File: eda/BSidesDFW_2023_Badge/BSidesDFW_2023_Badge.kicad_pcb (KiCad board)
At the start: 2 copper layers, 50 x 63 mm, 12 parts

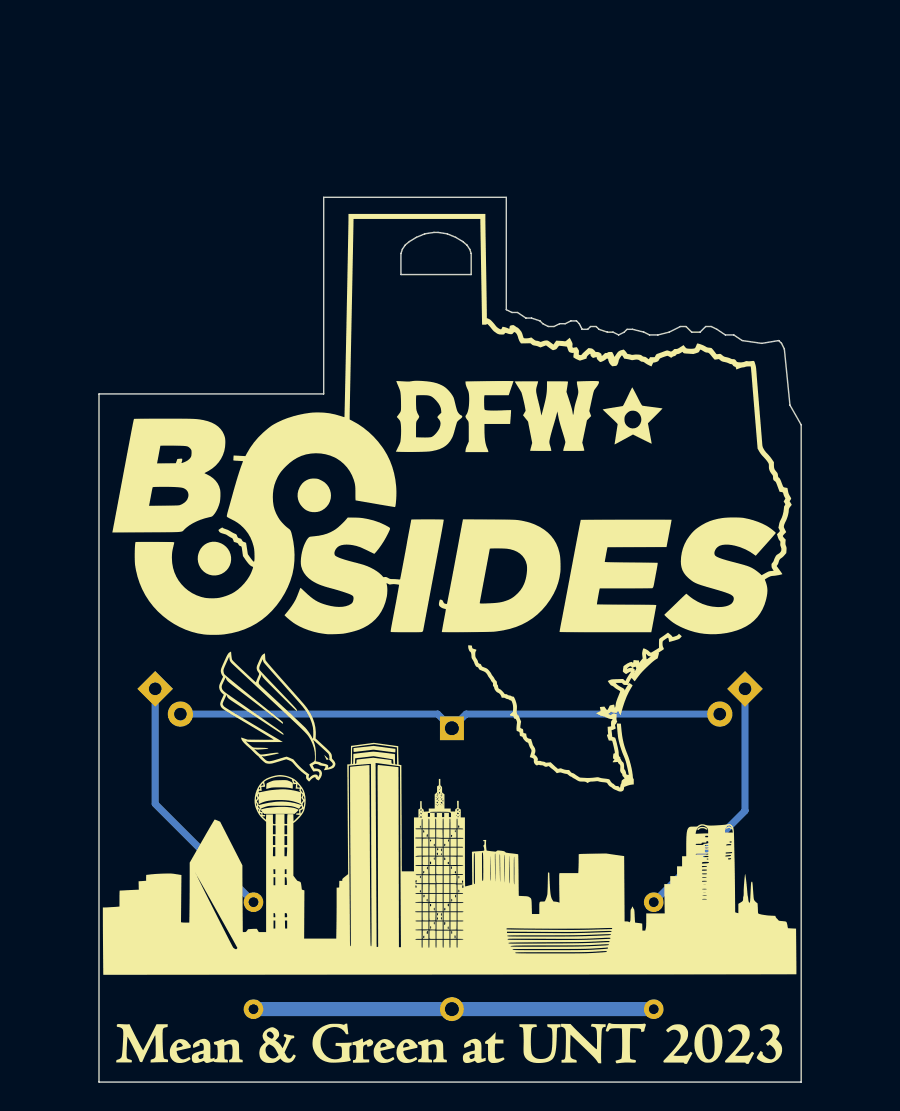
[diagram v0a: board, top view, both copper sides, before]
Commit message: final pcb design
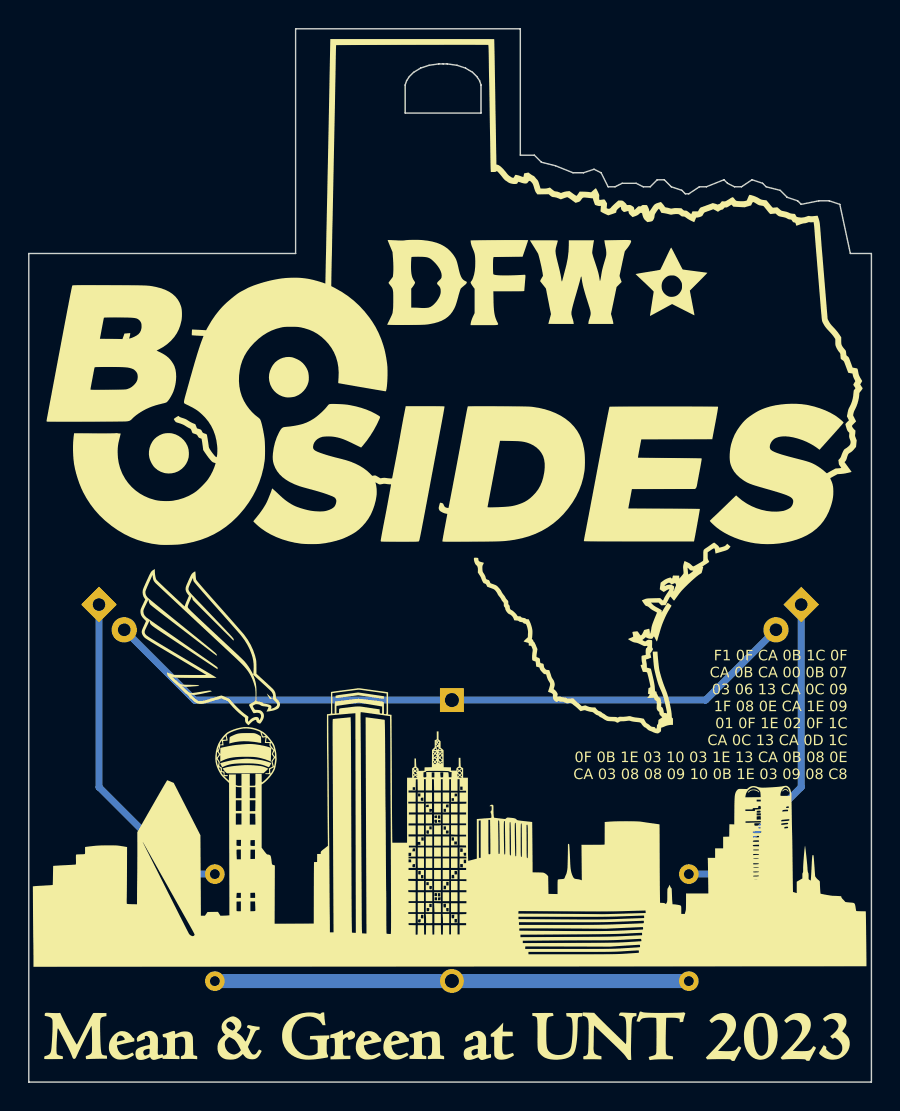
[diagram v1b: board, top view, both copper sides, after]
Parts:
- added G***: bsilk-scrappy, 0_local:0_UNT_old_scrappy_bsilk_1, F.Cu at (91.6, 127.6)
- BT1: footprint 0_local:BatteryHolder_CR2032-BS-2-1_Front_backsilk -> 0_local:BatteryHolder_CR2032-BS-2-1_Back_backsilk
- D1, D2: footprint 0_local:LED_D5.0mm-2_backsilk -> 0_local:LED_D5.0mm-2_backsilk_3Dback_horiz
- G***: footprint 0_alt_bier:logo-alt_bier-1100dpi-8x21mm-back -> 0_alt_bier:logo-alt_bier-900dpi-10x25mm-back
- G001: renamed from G002; footprint 0_local:0_BsidesDFW_top_fsilk_2 -> 0_local:0_BsidesDFW_top_fsilk_4
- G002: renamed from G001; footprint 0_local:0_BsidesDFW_bot_fsilk_3 -> 0_local:0_BsidesDFW_bot_fsilk_4
- G003: footprint 0_local:0_BsidesDFW_fmask_2 -> 0_local:0_BsidesDFW_fmask_4
- G004: footprint 0_local:0_BsidesDFW_bmask_2 -> 0_local:0_BsidesDFW_bmask_4
- R1, R2: footprint 0_local:R_Axial_DIN0207_L6.3mm_D2.5mm_P7.62mm_Horizontal_backsilk -> 0_local:R_Axial_DIN0207_L6.3mm_D2.5mm_P7.62mm_Horizontal_backsilk_3Dback
- moved REF** 7.24 mm to (95.2, 108.1)
- moved REF** 7.21 mm to (134.7, 108.1)
- moved D1 7.21 mm to (140.0, 106.0)
- moved D2 7.21 mm to (90.0, 106.0)
- moved G004 5.85 mm to (115.0, 102.5)
- moved G001 5.85 mm to (115.0, 102.5)
- moved G002 5.85 mm to (115.0, 102.5)
- moved G003 5.85 mm to (115.0, 102.5)
- moved G*** 4.27 mm to (138.0, 125.8)
- moved R2 3.40 mm to (98.2, 125.2)
- moved R1 3.20 mm to (132.0, 125.2)
- moved BT1 2.01 mm to (115.1, 135.8)
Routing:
- net Net-(BT1-Pad1): track 39.2 -> 50.6 mm
- net Net-(D2-Pad1): track 18.1 -> 23.8 mm
- net Net-(D1-Pad1): track 17.9 -> 23.6 mm
- net Net-(BT1-Pad2): track 28.5 -> 33.8 mm
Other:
- board size 50 x 63 mm -> 60 x 75 mm
- board text added: "Badge Details: https://bsidesdfw2023.altbier.us"
- board text added: "F1 0F CA 0B 1C 0F CA 0B CA 00 0B 07 03 06 13 CA 0C 09 1F 08 0E CA 1E 09 01 0F 1E 02 0F 1C CA 0C 13 CA 0D 1C 0F 0B 1E 03 10 03 1E 13 CA 0B 08 0E CA 03 08 08 09 10 0B 1E 03 09 08 C8"
- board text added: "Thanks to: Chelsea @romanescca for help with art, and Rex @r3x3r for moral support"
